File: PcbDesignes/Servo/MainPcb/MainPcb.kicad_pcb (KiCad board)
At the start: 2 copper layers, 45.2 x 42.6 mm, 13 parts, among them J1 Conn_02x02_Odd_Even, J2 Conn_01x04, J3 Conn_02x05_Odd_Even, J4 Conn_02x02_Odd_Even, J5 Conn_02x05_Odd_Even, J6 Conn_01x01, J7 Conn_01x01, J8 Conn_01x01, J9 Conn_01x01, U1 Itsybitsy, U2 TB6612FNG, U3 CurrentSensor

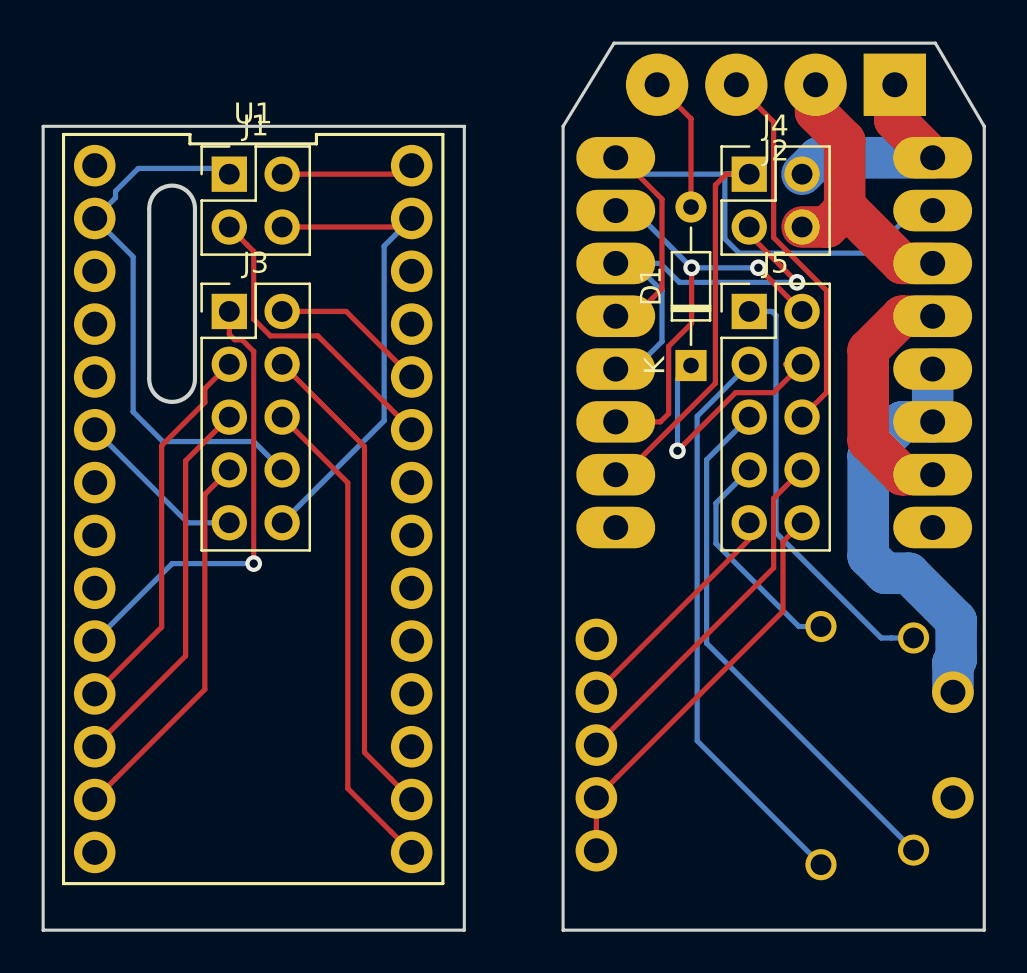
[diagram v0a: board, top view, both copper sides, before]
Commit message: updated schematics and PCB
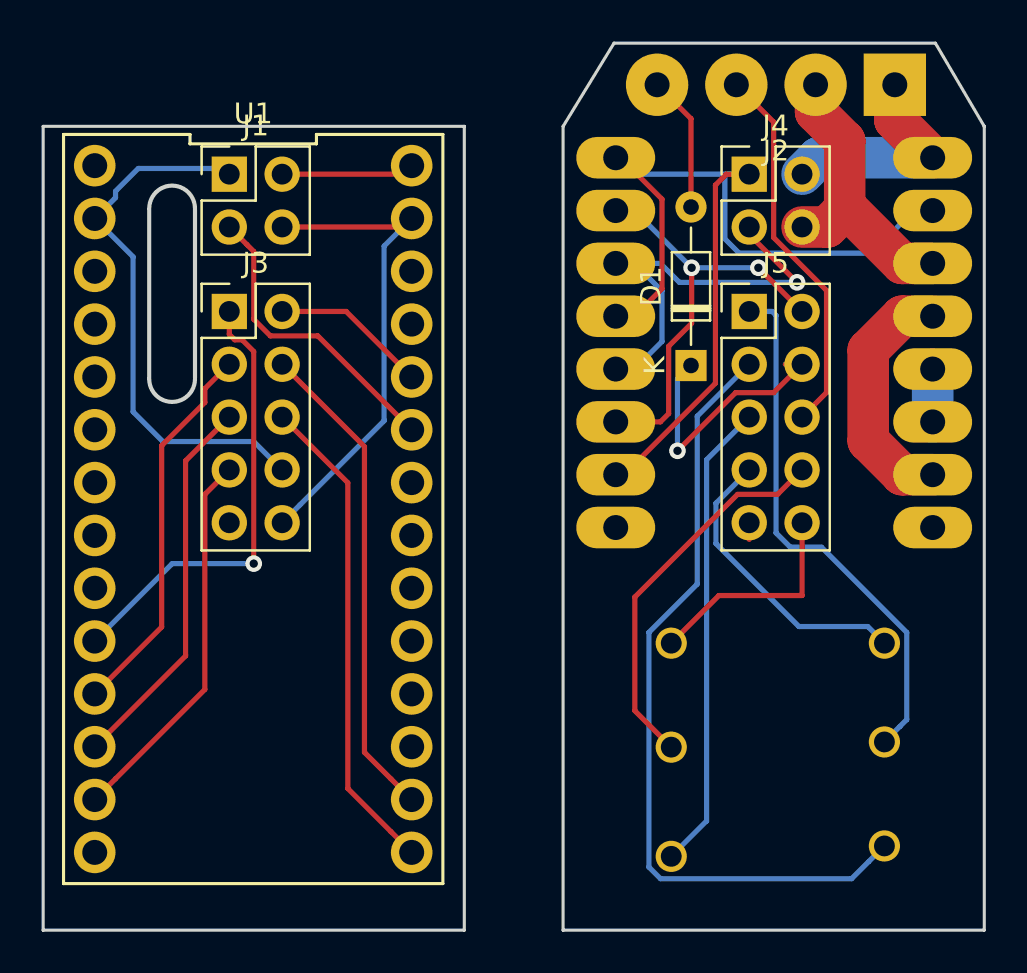
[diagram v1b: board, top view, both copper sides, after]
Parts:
- removed U3: CurrentSensor, Package_DIP:DIP-7_600_ELL
- added 3.3v1: Conn_01x01, Connector_Wire:SolderWirePad_1x01_Pad1.5mm_Drill1mm, B.Cu at (53.5, 52.5)
- added GND1: Conn_01x01, Connector_Wire:SolderWirePad_1x01_Pad1.5mm_Drill1mm, B.Cu at (53.5, 47.5)
- moved SI 11.7 mm to (53.5, 57.8)
- moved SC 5.19 mm to (63.8, 52.2)
- moved SCK 3.18 mm to (63.8, 57.2)
- moved SO 3.15 mm to (63.8, 47.5)
- renumbered J9 to SC, J8 to SCK, J7 to SI, J6 to SO
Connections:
- net Net-(U2-Pad4) renamed M-
- net Net-(U2-Pad5) renamed M+
- J3 pad 9: Net-(J3-Pad9) -> (no net)
- J5 pad 10: GND -> Net-(GND1-Pad1)
- J5 pad 8: +3V3 -> Net-(3.3v1-Pad1)
- J5 pad 9: Net-(J5-Pad9) -> (no net)
- U1 pad 1: Net-(U1-Pad1) -> (no net)
- U1 pad 14: Net-(U1-Pad14) -> (no net)
- U1 pad 17: Net-(U1-Pad17) -> (no net)
- U1 pad 18: Net-(U1-Pad18) -> (no net)
- U1 pad 19: Net-(U1-Pad19) -> (no net)
- U1 pad 20: Net-(U1-Pad20) -> (no net)
- U1 pad 21: Net-(U1-Pad21) -> (no net)
- U1 pad 22: Net-(U1-Pad22) -> (no net)
- U1 pad 25: Net-(U1-Pad25) -> (no net)
- U1 pad 26: Net-(U1-Pad26) -> (no net)
- U1 pad 3: Net-(U1-Pad3) -> (no net)
- U1 pad 4: Net-(U1-Pad4) -> (no net)
- U1 pad 5: Net-(U1-Pad5) -> (no net)
- U1 pad 6: Net-(J3-Pad9) -> (no net)
- U1 pad 7: Net-(U1-Pad7) -> (no net)
- U1 pad 8: Net-(U1-Pad8) -> (no net)
- U1 pad 9: Net-(U1-Pad9) -> (no net)
- U2 pad 8: Net-(U2-Pad8) -> (no net)
- U2 pad 9: Net-(U2-Pad9) -> (no net)
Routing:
- net GND: track 19.9 -> 0.00 mm
- net Net-(3.3v1-Pad1): track 0.00 -> 18.5 mm
- net M+: track 20.2 -> 2.54 mm
- net +3V3: track 17.3 -> 0.00 mm
- net Net-(J5-Pad9): track 11.2 -> 0.00 mm
- net Net-(J5-Pad3): track 27.6 -> 38.4 mm
- net Net-(GND1-Pad1): track 0.00 -> 10.7 mm
- net Net-(J3-Pad9): track 8.32 -> 0.00 mm
- net Net-(J5-Pad1): track 20.5 -> 25.8 mm
- net Net-(J5-Pad7): track 10.9 -> 14.3 mm
- net Net-(J5-Pad5): track 25.8 -> 22.7 mm
- net (no net): track 0.00 -> 0.80 mm
